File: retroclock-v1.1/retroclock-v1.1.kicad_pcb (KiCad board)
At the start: 4 copper layers, 147.5 x 108 mm, 22 parts, among them J1 Hours, J2 Mins, J3 Secs, J4 Nixie YY2, J5 Nixie YY1, J6 Nixie MM2, J7 Nixie MM1, J8 Nixie DD2, J9 Nixie DD1

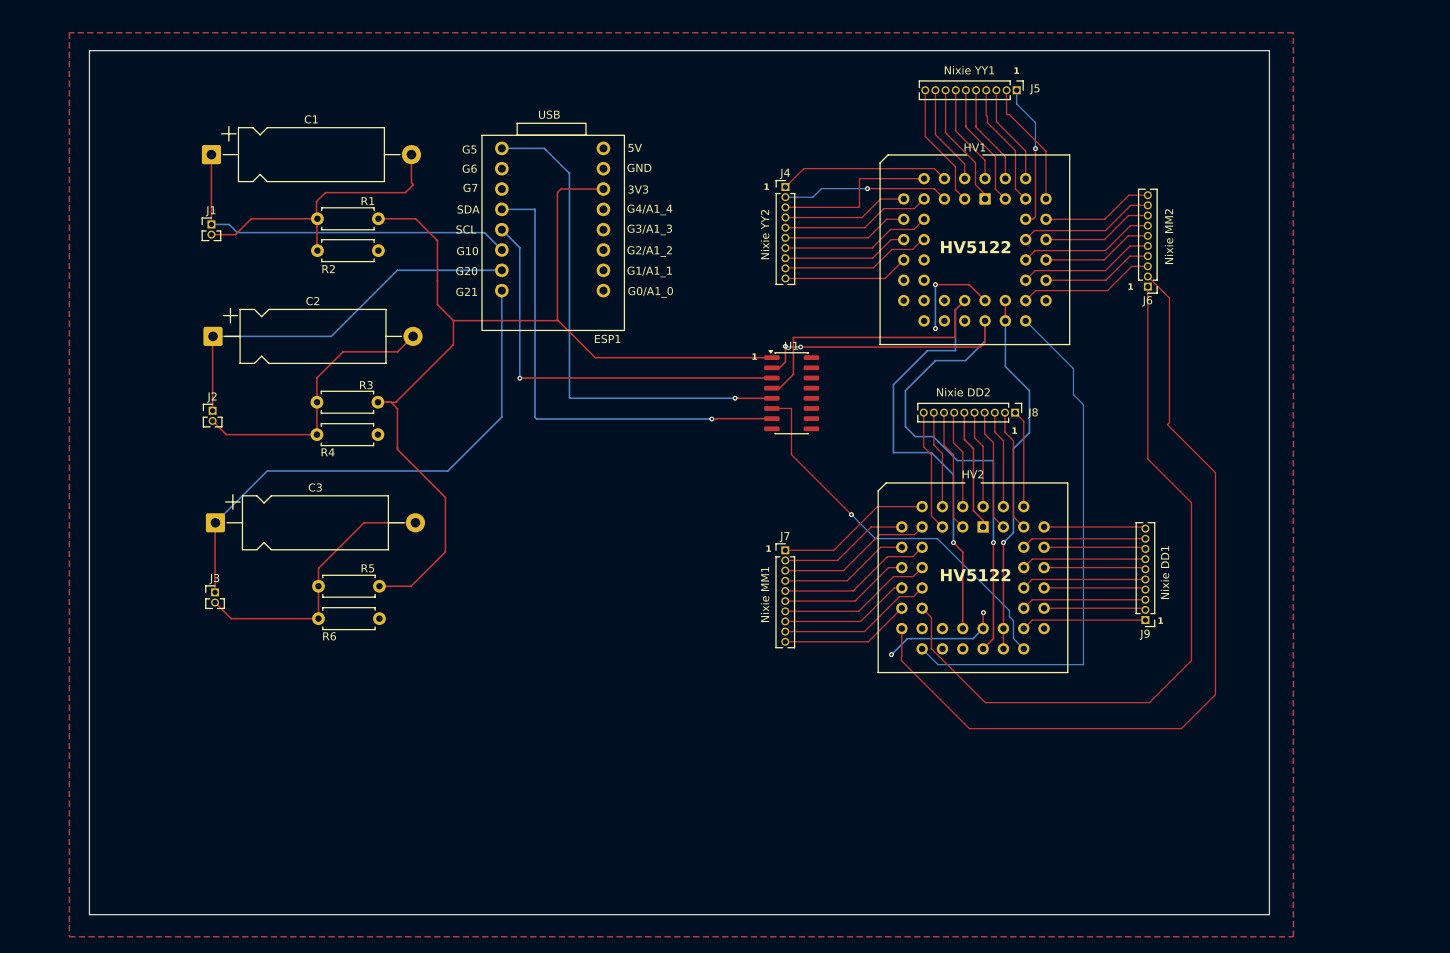
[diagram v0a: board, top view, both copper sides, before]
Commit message: retroclock 1.1 sent to JLCPCB!
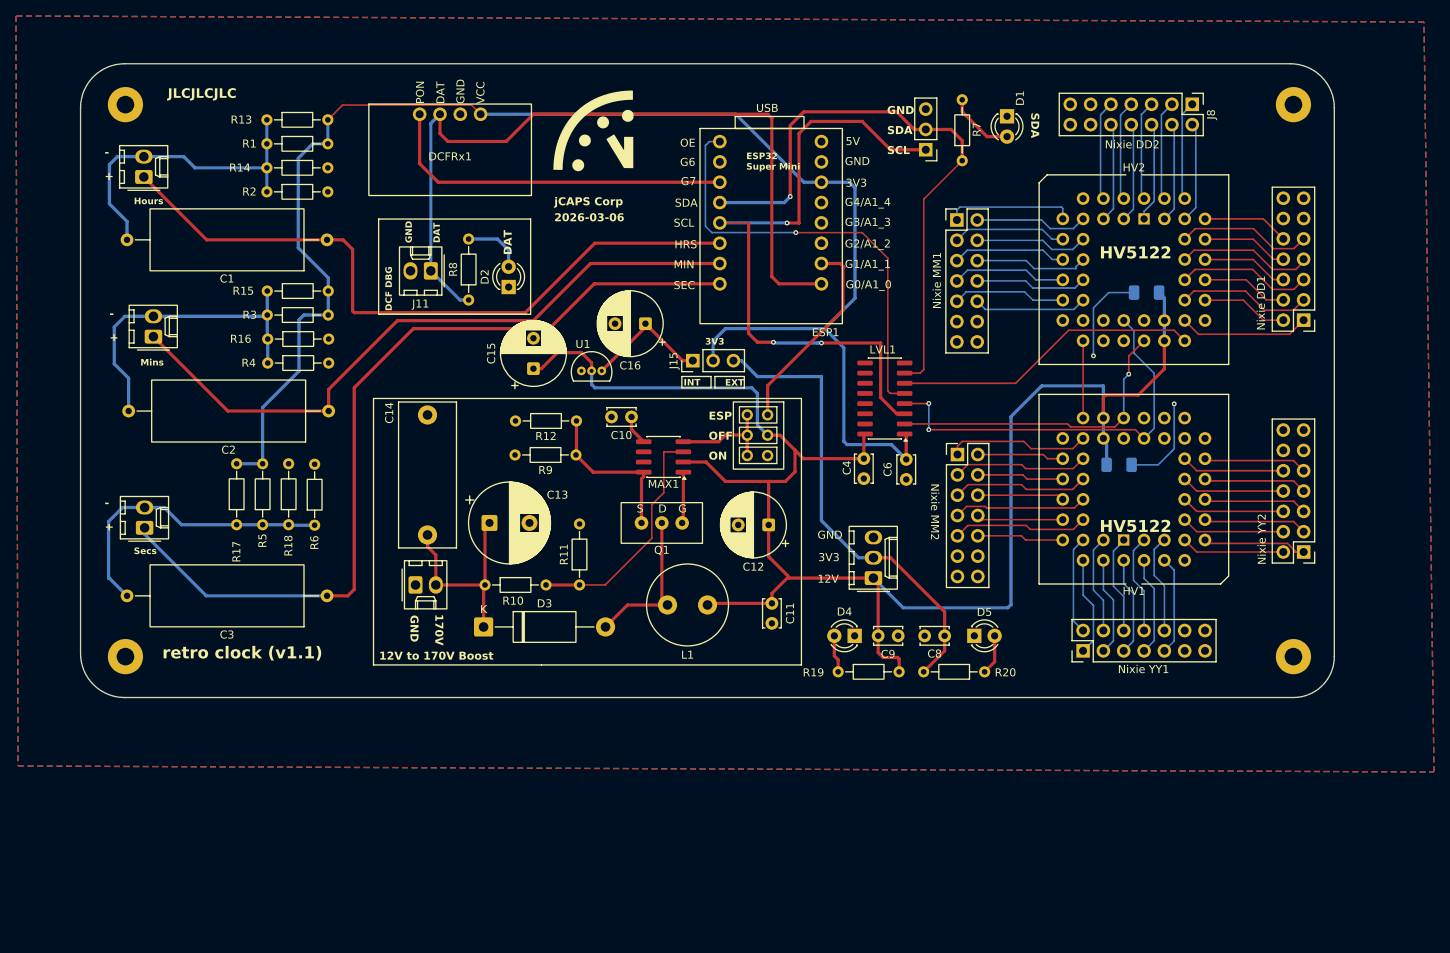
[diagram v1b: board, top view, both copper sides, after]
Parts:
- added C10: 100nF, Capacitor_THT:C_Disc_D3.4mm_W2.1mm_P2.50mm, F.Cu at (144.3, 84.0)
- added C11: 100nF, Capacitor_THT:C_Disc_D3.4mm_W2.1mm_P2.50mm, F.Cu at (161.8, 107.3)
- added C12: 68uF, Capacitor_THT:CP_Radial_D8.0mm_P3.80mm, F.Cu at (161.4, 97.5)
- added C13: 100uF, Capacitor_THT:CP_Radial_D10.0mm_P5.00mm, F.Cu at (126.5, 97.3)
- added C14: 100nF, Capacitor_THT:C_Rect_L18.0mm_W7.0mm_P15.00mm_FKS3_FKP3, F.Cu at (118.8, 98.8)
- added C15: 10uF, Capacitor_THT:CP_Radial_D8.0mm_P3.80mm, F.Cu at (132.0, 78.0)
- added C16: 10uF, Capacitor_THT:CP_Radial_D8.0mm_P3.80mm, F.Cu at (146.0, 72.4)
- added C4: 100n, Capacitor_THT:C_Disc_D3.4mm_W2.1mm_P2.50mm, F.Cu at (173.3, 89.2)
- added C5: 100n, Capacitor_SMD:C_1206_3216Metric_Pad1.33x1.80mm_HandSolder, B.Cu at (205.2, 90.0)
- added C6: 100n, Capacitor_THT:C_Disc_D3.4mm_W2.1mm_P2.50mm, F.Cu at (178.6, 91.8)
- added C7: 100n, Capacitor_SMD:C_1206_3216Metric_Pad1.33x1.80mm_HandSolder, B.Cu at (208.7, 68.5)
- added C8: 100n, Capacitor_THT:C_Disc_D3.4mm_W2.1mm_P2.50mm, F.Cu at (183.4, 111.4)
- added C9: 100n, Capacitor_THT:C_Disc_D3.4mm_W2.1mm_P2.50mm, F.Cu at (177.6, 111.4)
- added D1: LED, LED_THT:LED_D3.0mm_Clear, F.Cu at (191.2, 46.5)
- added D2: LED, LED_THT:LED_D3.0mm_Clear, F.Cu at (128.9, 67.8)
- added D3: RF01VM2S, Diode_THT:D_DO-15_P15.24mm_Horizontal, F.Cu at (125.8, 110.3)
- added D4: LED, LED_THT:LED_D3.0mm_Clear, F.Cu at (172.2, 111.4)
- added D5: LED, LED_THT:LED_D3.0mm_Clear, F.Cu at (187.1, 111.4)
- added DCFRx1: ~, 01_mjc_library:DCF77Rx_A, F.Cu at (121.6, 50.0)
- added G***: LOGO, 01_mjc_library:doomsday_clock, F.Cu at (139.5, 48.3)
- added H1: MountingHole, MountingHole:MountingHole_2.2mm_M2_Pad, F.Cu at (81.0, 45.0)
- added H2: MountingHole, MountingHole:MountingHole_2.2mm_M2_Pad, F.Cu at (81.0, 114.0)
- added H3: MountingHole, MountingHole:MountingHole_2.2mm_M2_Pad, F.Cu at (227.0, 45.0)
- added H4: MountingHole, MountingHole:MountingHole_2.2mm_M2_Pad, F.Cu at (227.0, 114.0)
- added J10: Serial DBG, Connector_PinHeader_2.54mm:PinHeader_1x03_P2.54mm_Vertical, F.Cu at (181.0, 50.6)
- added J11: DCF DBG, Connector_Molex:Molex_KK-254_AE-6410-02A_1x02_P2.54mm_Vertical, F.Cu at (119.2, 65.8)
- added J12: Supply, Connector_Molex:Molex_KK-254_AE-6410-03A_1x03_P2.54mm_Vertical, F.Cu at (174.5, 104.2)
- added J13: 170V, Connector_Molex:Molex_KK-254_AE-6410-02A_1x02_P2.54mm_Vertical, F.Cu at (117.3, 105.0)
- added J14: ~, 01_mjc_library:Jumper 2.54 2x03, F.Cu at (160.0, 86.4)
- added J15: 3v3 src, Connector_PinHeader_2.54mm:PinHeader_1x03_P2.54mm_Vertical, F.Cu at (151.9, 77.0)
- added L1: 100H, Inductor_THT:L_Radial_D10.0mm_P5.00mm_Neosid_SD12k_style3, F.Cu at (153.8, 107.5)
- added LVL1: ~, Package_SO:SOIC-16_3.9x9.9mm_P1.27mm, F.Cu at (175.9, 81.7)
- added MAX1: MAX1771, Package_SO:SOIC-8_3.9x4.9mm_P1.27mm, F.Cu at (148.3, 89.0)
- added Q1: ~, 01_mjc_library:MOSFET, F.Cu at (148.1, 97.3)
- added R10: 1.2M, Resistor_THT:R_Axial_DIN0204_L3.6mm_D1.6mm_P7.62mm_Horizontal, F.Cu at (126.0, 105.0)
- added R11: 10k, Resistor_THT:R_Axial_DIN0204_L3.6mm_D1.6mm_P7.62mm_Horizontal, F.Cu at (137.8, 105.0)
- added R12: 0.2, Resistor_THT:R_Axial_DIN0204_L3.6mm_D1.6mm_P7.62mm_Horizontal, F.Cu at (137.4, 84.5)
- added R13: R, Resistor_THT:R_Axial_DIN0204_L3.6mm_D1.6mm_P7.62mm_Horizontal, F.Cu at (98.7, 46.9)
- added R14: R, Resistor_THT:R_Axial_DIN0204_L3.6mm_D1.6mm_P7.62mm_Horizontal, F.Cu at (98.7, 52.9)
- added R15: R, Resistor_THT:R_Axial_DIN0204_L3.6mm_D1.6mm_P7.62mm_Horizontal, F.Cu at (98.7, 68.3)
- added R16: R, Resistor_THT:R_Axial_DIN0204_L3.6mm_D1.6mm_P7.62mm_Horizontal, F.Cu at (98.8, 74.3)
- added R17: R, Resistor_THT:R_Axial_DIN0204_L3.6mm_D1.6mm_P7.62mm_Horizontal, F.Cu at (94.9, 97.5)
- added R18: R, Resistor_THT:R_Axial_DIN0204_L3.6mm_D1.6mm_P7.62mm_Horizontal, F.Cu at (101.4, 97.5)
- added R19: R, Resistor_THT:R_Axial_DIN0204_L3.6mm_D1.6mm_P7.62mm_Horizontal, F.Cu at (170.1, 115.9)
- added R20: R, Resistor_THT:R_Axial_DIN0204_L3.6mm_D1.6mm_P7.62mm_Horizontal, F.Cu at (188.4, 115.9)
- added R7: R, Resistor_THT:R_Axial_DIN0204_L3.6mm_D1.6mm_P7.62mm_Horizontal, F.Cu at (185.6, 52.0)
- added R8: R, Resistor_THT:R_Axial_DIN0204_L3.6mm_D1.6mm_P7.62mm_Horizontal, F.Cu at (123.9, 69.4)
- added R9: 0.2, Resistor_THT:R_Axial_DIN0204_L3.6mm_D1.6mm_P7.62mm_Horizontal, F.Cu at (137.3, 88.8)
- C1, C2, C3: footprint Capacitor_THT:CP_Axial_L18.0mm_D6.5mm_P25.00mm_Horizontal -> Capacitor_THT:C_Axial_L19.0mm_D7.5mm_P25.00mm_Horizontal
- ESP1: footprint mjc_library:ESP32 Header -> 01_mjc_library:ESP32 Header
- HV1, HV2: footprint mjc_library:PLCC-44_THT-Socket -> 01_mjc_library:PLCC44 MillMaxMfg 940
- J1, J2, J3: footprint Connector_PinHeader_1.27mm:PinHeader_1x02_P1.27mm_Vertical -> Connector_Molex:Molex_KK-254_AE-6410-02A_1x02_P2.54mm_Vertical
- J4, J6, J7, J8: footprint Connector_PinHeader_1.27mm:PinHeader_1x10_P1.27mm_Vertical -> Connector_PinHeader_2.54mm:PinHeader_2x07_P2.54mm_Vertical
- J5: value Nixie YY1 -> Nixie DD1; footprint Connector_PinHeader_1.27mm:PinHeader_1x10_P1.27mm_Vertical -> Connector_PinHeader_2.54mm:PinHeader_2x07_P2.54mm_Vertical
- J9: value Nixie DD1 -> Nixie YY1; footprint Connector_PinHeader_1.27mm:PinHeader_1x10_P1.27mm_Vertical -> Connector_PinHeader_2.54mm:PinHeader_2x07_P2.54mm_Vertical
- R1, R2, R3, R4, R5, R6: footprint Resistor_THT:R_Axial_DIN0207_L6.3mm_D2.5mm_P7.62mm_Horizontal -> Resistor_THT:R_Axial_DIN0204_L3.6mm_D1.6mm_P7.62mm_Horizontal
- U1: footprint Package_SO:SOIC-16_3.9x9.9mm_P1.27mm -> 01_mjc_library:HT7333
- moved J4 79.2 mm to (228.3, 100.9), turned to 180 degrees
- moved J7 46.5 mm to (184.9, 59.4)
- moved HV1 46.0 mm to (205.8, 99.4), turned to 180 degrees
- moved J5 46.0 mm to (228.3, 71.9), turned to 180 degrees
- moved J8 44.4 mm to (214.3, 45.0)
- moved HV2 43.4 mm to (208.3, 59.3)
- moved J6 31.7 mm to (185.0, 88.7), turned to 0 degrees
- moved ESP1 27.3 mm to (162.9, 59.8)
- moved U1 25.2 mm to (139.3, 78.3)
- moved C1 18.0 mm to (106.2, 61.9), turned to 180 degrees
- moved C2 17.2 mm to (106.4, 83.3), turned to 180 degrees
- moved C3 16.7 mm to (106.2, 106.4), turned to 180 degrees
- moved R3 12.5 mm to (98.7, 71.3)
- moved J3 11.9 mm to (83.4, 97.9), turned to 90 degrees
- moved J2 11.9 mm to (84.5, 74.0), turned to 90 degrees
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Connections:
- net Net-(ESP1-G10) renamed AM_HRS
- net Net-(ESP1-G20) renamed AM_MIN
- net Net-(ESP1-G21) renamed AM_SEC
- net Net-(J1-Pin_2) renamed /ammeter_driver/AM_H-
- net Net-(J2-Pin_2) renamed /ammeter_driver/AM_M-
- net Net-(J3-Pin_2) renamed /ammeter_driver/AM_S-
- ESP1 pad 1: Net-(ESP1-G5) -> /OE
- ESP1 pad 10: unconnected-(ESP1-G1/A1_1-Pad10) -> /BOOST_EN
- ESP1 pad 3: unconnected-(ESP1-G7-Pad3) -> DCF_PON
- ESP1 pad 4: Net-(ESP1-SDA) -> /SDA
- ESP1 pad 5: Net-(ESP1-SCL) -> /SCL
- ESP1 pad 9: unconnected-(ESP1-G0/A1_0-Pad9) -> DCF_DAT
- HV1 pad 1: Net-(HL1-HVO16) -> Net-(HV1-HVO16)
- HV1 pad 10: Net-(HL1-HVO25) -> Net-(HV1-HVO25)
- HV1 pad 11: Net-(HL1-HVO26) -> Net-(HV1-HVO26)
- HV1 pad 12: Net-(HL1-HVO27) -> Net-(HV1-HVO27)
- HV1 pad 13: Net-(HL1-HVO28) -> Net-(HV1-HVO28)
- HV1 pad 14: unconnected-(HL1-HVO29-Pad14) -> Net-(HV1-HVO29)
- HV1 pad 15: unconnected-(HL1-HVO30-Pad15) -> Net-(HV1-HVO30)
- HV1 pad 16: unconnected-(HL1-HVO31-Pad16) -> Net-(HV1-HVO31)
- HV1 pad 2: Net-(HL1-HVO17) -> Net-(HV1-HVO17)
- HV1 pad 23: Net-(HL1-OE) -> NIX_OE
- HV1 pad 24: Net-(HL1-CLK) -> NIX_CLK
- HV1 pad 3: Net-(HL1-HVO18) -> Net-(HV1-HVO18)
- HV1 pad 30: Net-(HL1-HVO1) -> Net-(HV1-HVO1)
- HV1 pad 31: Net-(HL1-HVO2) -> Net-(HV1-HVO2)
- HV1 pad 32: Net-(HL1-HVO3) -> Net-(HV1-HVO3)
- HV1 pad 33: Net-(HL1-HVO4) -> Net-(HV1-HVO4)
- HV1 pad 34: Net-(HL1-HVO5) -> Net-(HV1-HVO5)
- HV1 pad 35: Net-(HL1-HVO6) -> Net-(HV1-HVO6)
- HV1 pad 36: Net-(HL1-HVO7) -> Net-(HV1-HVO7)
- HV1 pad 37: Net-(HL1-HVO8) -> Net-(HV1-HVO8)
- HV1 pad 38: Net-(HL1-HVO9) -> Net-(HV1-HVO9)
- HV1 pad 39: Net-(HL1-HVO10) -> Net-(HV1-HVO10)
- HV1 pad 4: Net-(HL1-HVO19) -> Net-(HV1-HVO19)
- HV1 pad 40: Net-(HL1-HVO11) -> Net-(HV1-HVO11)
- HV1 pad 41: Net-(HL1-HVO12) -> Net-(HV1-HVO12)
- HV1 pad 42: Net-(HL1-HVO13) -> Net-(HV1-HVO13)
- HV1 pad 43: Net-(HL1-HVO14) -> Net-(HV1-HVO14)
- HV1 pad 44: Net-(HL1-HVO15) -> Net-(HV1-HVO15)
- HV1 pad 5: Net-(HL1-HVO20) -> Net-(HV1-HVO20)
- HV1 pad 6: Net-(HL1-HVO21) -> unconnected-(HV1-HVO21-Pad6)
- HV1 pad 7: Net-(HL1-HVO22) -> Net-(HV1-HVO22)
- HV1 pad 8: Net-(J4-Pin_5) -> Net-(HV1-HVO23)
- HV1 pad 9: Net-(HL1-HVO24) -> Net-(HV1-HVO24)
- HV2 pad 10: Net-(HL2-HVO25) -> Net-(HV2-HVO25)
- HV2 pad 11: Net-(HL2-HVO26) -> Net-(HV2-HVO26)
- HV2 pad 12: Net-(HL2-HVO27) -> Net-(HV2-HVO27)
- HV2 pad 13: Net-(HL2-HVO28) -> Net-(HV2-HVO28)
- HV2 pad 14: Net-(HL2-HVO29) -> Net-(HV2-HVO29)
- HV2 pad 15: Net-(HL2-HVO30) -> Net-(HV2-HVO30)
- HV2 pad 16: Net-(HL2-HVO31) -> Net-(HV2-HVO31)
- HV2 pad 17: Net-(J6-Pin_2) -> unconnected-(HV2-HVO32-Pad17)
- HV2 pad 23: Net-(HL1-OE) -> NIX_OE
- HV2 pad 24: Net-(HL1-CLK) -> NIX_CLK
- HV2 pad 28: Net-(HL2-D_IN) -> NIX_DAT_IN
- HV2 pad 30: Net-(HL2-HVO1) -> Net-(HV2-HVO1)
- HV2 pad 31: Net-(HL2-HVO2) -> Net-(HV2-HVO2)
- HV2 pad 32: Net-(HL2-HVO3) -> Net-(HV2-HVO3)
- HV2 pad 33: Net-(HL2-HVO4) -> Net-(HV2-HVO4)
- HV2 pad 34: Net-(HL2-HVO5) -> Net-(HV2-HVO5)
- HV2 pad 35: Net-(HL2-HVO6) -> Net-(HV2-HVO6)
- HV2 pad 36: Net-(HL2-HVO7) -> Net-(HV2-HVO7)
- HV2 pad 37: Net-(HL2-HVO8) -> Net-(HV2-HVO8)
- HV2 pad 38: Net-(HL2-HVO9) -> Net-(HV2-HVO9)
- HV2 pad 39: Net-(HL2-HVO10) -> Net-(HV2-HVO10)
- HV2 pad 6: Net-(HL2-HVO21) -> unconnected-(HV2-HVO21-Pad6)
- HV2 pad 7: Net-(HL2-HVO22) -> Net-(HV2-HVO22)
- HV2 pad 8: Net-(J7-Pin_3) -> Net-(HV2-HVO23)
- HV2 pad 9: Net-(HL2-HVO24) -> Net-(HV2-HVO24)
- J4 pad 1: Net-(HL1-HVO19) -> Net-(HV1-HVO22)
- J4 pad 10: Net-(HL1-HVO28) -> Net-(HV1-HVO31)
- J4 pad 2: Net-(HL1-HVO20) -> Net-(HV1-HVO23)
- J4 pad 3: Net-(HL1-HVO21) -> Net-(HV1-HVO24)
- J4 pad 4: Net-(HL1-HVO22) -> Net-(HV1-HVO25)
- J4 pad 5: Net-(J4-Pin_5) -> Net-(HV1-HVO26)
- J4 pad 6: Net-(HL1-HVO24) -> Net-(HV1-HVO27)
- J4 pad 7: Net-(HL1-HVO25) -> Net-(HV1-HVO28)
- J4 pad 8: Net-(HL1-HVO26) -> Net-(HV1-HVO29)
- J4 pad 9: Net-(HL1-HVO27) -> Net-(HV1-HVO30)
- J5 pad 1: Net-(HL1-HVO9) -> Net-(HV2-HVO1)
- J5 pad 10: Net-(HL1-HVO18) -> Net-(HV2-HVO10)
- J5 pad 2: Net-(HL1-HVO10) -> Net-(HV2-HVO2)
- J5 pad 3: Net-(HL1-HVO11) -> Net-(HV2-HVO3)
- J5 pad 4: Net-(HL1-HVO12) -> Net-(HV2-HVO4)
- J5 pad 5: Net-(HL1-HVO13) -> Net-(HV2-HVO5)
- J5 pad 6: Net-(HL1-HVO14) -> Net-(HV2-HVO6)
- J5 pad 7: Net-(HL1-HVO15) -> Net-(HV2-HVO7)
- J5 pad 8: Net-(HL1-HVO16) -> Net-(HV2-HVO8)
- J5 pad 9: Net-(HL1-HVO17) -> Net-(HV2-HVO9)
- J6 pad 1: Net-(HL2-HVO31) -> Net-(HV1-HVO1)
- J6 pad 10: Net-(HL1-HVO8) -> Net-(HV1-HVO10)
- J6 pad 2: Net-(J6-Pin_2) -> Net-(HV1-HVO2)
- J6 pad 3: Net-(HL1-HVO1) -> Net-(HV1-HVO3)
- J6 pad 4: Net-(HL1-HVO2) -> Net-(HV1-HVO4)
- J6 pad 5: Net-(HL1-HVO3) -> Net-(HV1-HVO5)
- J6 pad 6: Net-(HL1-HVO4) -> Net-(HV1-HVO6)
- J6 pad 7: Net-(HL1-HVO5) -> Net-(HV1-HVO7)
- J6 pad 8: Net-(HL1-HVO6) -> Net-(HV1-HVO8)
- J6 pad 9: Net-(HL1-HVO7) -> Net-(HV1-HVO9)
- J7 pad 1: Net-(HL2-HVO21) -> Net-(HV2-HVO22)
- J7 pad 10: Net-(HL2-HVO30) -> Net-(HV2-HVO31)
- J7 pad 2: Net-(HL2-HVO22) -> Net-(HV2-HVO23)
- J7 pad 3: Net-(J7-Pin_3) -> Net-(HV2-HVO24)
- J7 pad 4: Net-(HL2-HVO24) -> Net-(HV2-HVO25)
- J7 pad 5: Net-(HL2-HVO25) -> Net-(HV2-HVO26)
- J7 pad 6: Net-(HL2-HVO26) -> Net-(HV2-HVO27)
- J7 pad 7: Net-(HL2-HVO27) -> Net-(HV2-HVO28)
- J7 pad 8: Net-(HL2-HVO28) -> Net-(HV2-HVO29)
- J7 pad 9: Net-(HL2-HVO29) -> Net-(HV2-HVO30)
- J9 pad 1: Net-(HL2-HVO1) -> Net-(HV1-HVO11)
- J9 pad 10: Net-(HL2-HVO10) -> Net-(HV1-HVO20)
- J9 pad 2: Net-(HL2-HVO2) -> Net-(HV1-HVO12)
- J9 pad 3: Net-(HL2-HVO3) -> Net-(HV1-HVO13)
- J9 pad 4: Net-(HL2-HVO4) -> Net-(HV1-HVO14)
- J9 pad 5: Net-(HL2-HVO5) -> Net-(HV1-HVO15)
- J9 pad 6: Net-(HL2-HVO6) -> Net-(HV1-HVO16)
- J9 pad 7: Net-(HL2-HVO7) -> Net-(HV1-HVO17)
- J9 pad 8: Net-(HL2-HVO8) -> Net-(HV1-HVO18)
- J9 pad 9: Net-(HL2-HVO9) -> Net-(HV1-HVO19)
- U1 pad 1: +3V3 -> GND
- U1 pad 2: Net-(HL1-CLK) -> +12V
- U1 pad 3: Net-(ESP1-SCL) -> Net-(J15-Pin_1)
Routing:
- net +12V: track 46.1 -> 209.9 mm, vias 1 -> 0
- net Net-(J6-Pin_2): track 104.5 -> 0.00 mm
- net DCF_DAT: track 0.00 -> 98.6 mm
- net Net-(HL2-HVO31): track 92.0 -> 0.00 mm
- net Net-(HL1-CLK): track 88.3 -> 0.00 mm, vias 3 -> 0
- net Net-(HL1-OE): track 86.5 -> 0.00 mm, vias 1 -> 0
- net /SCL: track 0.00 -> 84.1 mm, vias 0 -> 3
- net /SDA: track 0.00 -> 74.9 mm, vias 0 -> 1
- net Net-(ESP1-G5): track 63.2 -> 0.00 mm, vias 1 -> 0
- net Net-(ESP1-SDA): track 59.9 -> 0.00 mm, vias 1 -> 0
- net Net-(J12-Pin_2): track 0.00 -> 58.5 mm
- net +3V3: track 131.7 -> 189.9 mm
- net Net-(HV1-D_IN): track 66.9 -> 9.66 mm
- net /OE: track 0.00 -> 55.4 mm, vias 0 -> 1
- net Net-(ESP1-SCL): track 51.0 -> 0.00 mm, vias 1 -> 0
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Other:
- board size 147.5 x 108 mm -> 156.7 x 79.2 mm
- copper layers 4 -> 2
- board text added: "+"
- board text added: "-"
- board text added: "12V"
- board text added: "12V to 170V Boost"
- board text added: "170V"
- board text added: "2026-03-06"
- board text added: "3V3"
- board text added: "DAT"
- board text added: "DCF DBG"
- board text added: "ESP"
- board text added: "ESP32 Super Mini"
- board text added: "EXT"
- board text added: "GND"
- board text added: "Hours"
- board text added: "INT"
- board text added: "JLCJLCJLC"
- board text added: "Mins"
- board text added: "OFF"
- board text added: "ON"
- board text added: "SCL"
- board text added: "SDA"
- board text added: "Secs"
- board text added: "jCAPS Corp"
- board text added: "retro clock (v1.1)"
- board text removed: "1"
